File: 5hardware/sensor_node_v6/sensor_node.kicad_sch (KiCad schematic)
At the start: 71 parts, among them J1 USB_C_Receptacle_USB2.0, J2 PJ-320D-A, J3 Conn_01x18_Socket, J4 Conn_01x18_Socket, J5 Conn_01x04_Pin, P1 S3B-PH-SM4-TB, Q1 BC818, Q2 Si2371EDS, Q3 AO3400A, Q4 Si2371EDS, Q5 Si2371EDS, SW1 SW_Push, SW2 RotaryEncoder, SW3 SW_Push, SW4 SW_Push, SW5 SW_Push, SW7 SW_Push, U1 INA219AxD, U12 APDS-9960, U13 SHT31-DIS, U15 DS1307Z+, U16 DS3231M, U17 BH1750FVI-TR, U2 ESP-12F, U4 CH32V003F4P6, U7 XC6206PxxxMR, U8 TPL5110, Y1 Crystal, Y2 Crystal

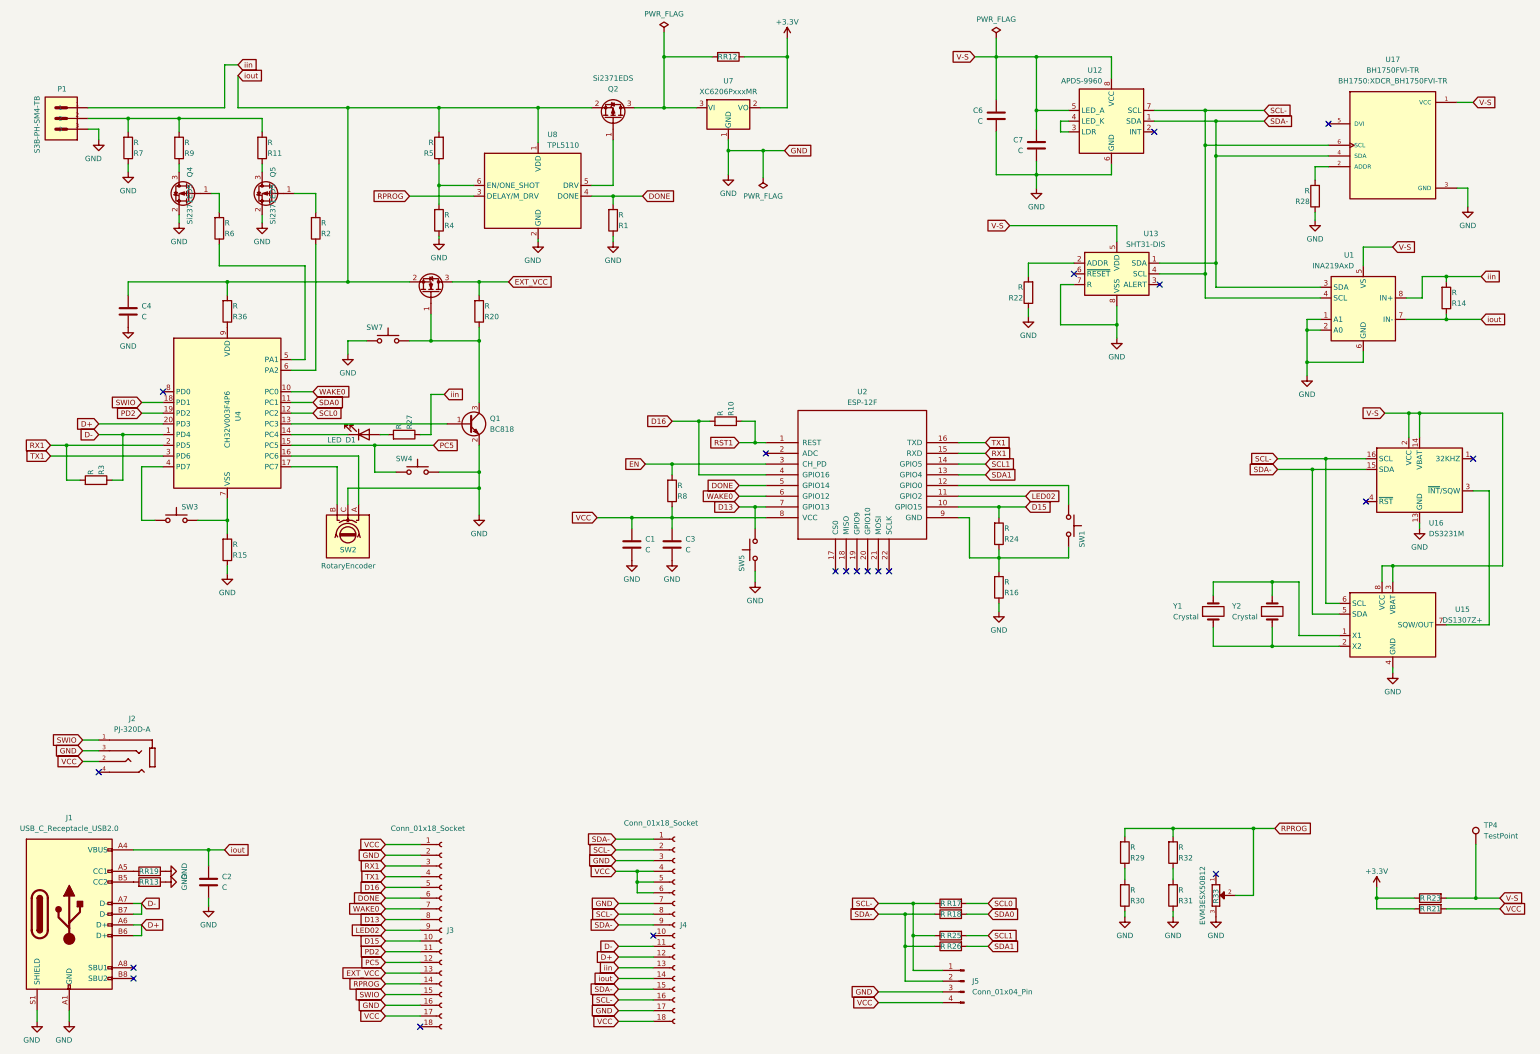
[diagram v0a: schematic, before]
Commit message: update PCB v8.0
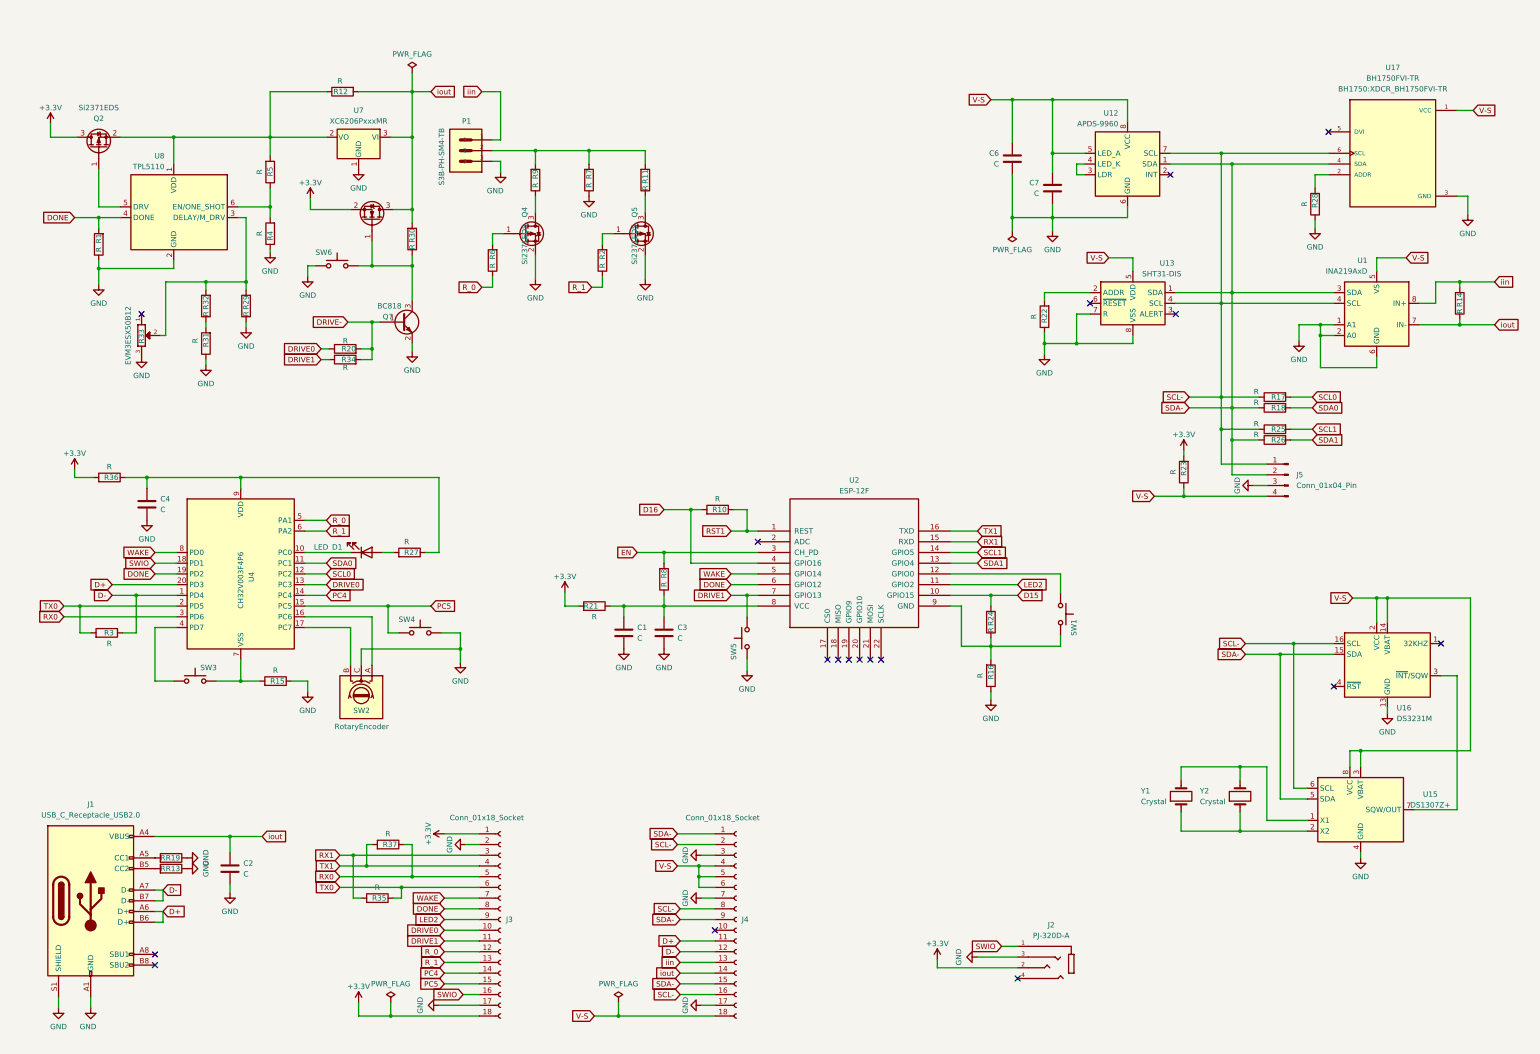
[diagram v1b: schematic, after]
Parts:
- removed Q1: BC818, Package_TO_SOT_SMD:SOT-23, symbol Transistor_BJT:BC818
- removed Q3: AO3400A, Package_TO_SOT_SMD:SOT-23, symbol Transistor_FET:AO3400A
- removed SW7: SW_Push, Button_Switch_SMD:SW_SPST_PTS810, symbol Switch:SW_Push
- removed TP4: TestPoint, Connector_PinHeader_1.00mm:PinHeader_1x01_P1.00mm_Vertical, symbol Connector:TestPoint
- added Q6: AO3400A, Package_TO_SOT_SMD:SOT-23, symbol Transistor_FET:AO3400A
- added Q7: BC818, Package_TO_SOT_SMD:SOT-23, symbol Transistor_BJT:BC818
- added R34, R35, R37: R, Resistor_SMD:R_0603_1608Metric, symbol Device:R
- added SW6: SW_Push, Button_Switch_SMD:SW_SPST_PTS810, symbol Switch:SW_Push
- C1, C2, C3, C4, C6, C7: footprint Capacitor_SMD:C_0805_2012Metric -> Capacitor_SMD:C_0603_1608Metric
- R1, R11, R13, R19, R2, R20, R24, R27, R29, R3, R30, R6, R7, R8, R9: footprint Resistor_SMD:R_0805_2012Metric -> Resistor_SMD:R_0603_1608Metric
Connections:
- net +3.3V: now also J2.2, J3.1 (Pin_1), J3.18 (Pin_18), Q2.3 (D), R21.2, R23.2, R36.2, Q6.2 (S); no longer R12.1, R21.1, R23.1, U7.2 (VO)
- net D+: now also J4.11 (Pin_11); no longer J4.12 (Pin_12)
- net D-: now also J4.12 (Pin_12); no longer J4.11 (Pin_11)
- net D15: no longer J3.10 (Pin_10)
- net D16: no longer J3.5 (Pin_5)
- net DONE: now also J3.8 (Pin_8), U2.6 (GPIO12), U4.19 (PD2); no longer J3.6 (Pin_6), U2.5 (GPIO14)
- net GND: now also J3.17 (Pin_17), R29.1, Q7.2 (E), SW6.1; no longer J3.16 (Pin_16), R30.1
- net PC5: now also J3.15 (Pin_15); no longer J3.12 (Pin_12)
- net RX1: now also R35.2; no longer R3.2, U4.2 (PD5)
- net SWIO: now also J3.16 (Pin_16); no longer J3.15 (Pin_15)
- net TX1: now also R37.2; no longer U4.3 (PD6)
- net V-S: now also J4.18 (Pin_18), J4.4 (Pin_4), J4.5 (Pin_5), J4.6 (Pin_6), J5.4 (Pin_4), R23.1; no longer R23.2
- net iin: no longer R27.1
- net iout: now also R12.2, R30.2, U7.3 (VI), Q6.3 (D); no longer C4.1, Q2.2 (S), R36.2, R5.2, U8.1 (VDD)
- net R_1: now reaches R2.1, U4.6 (PA2)
- net R_1: now also J3.13 (Pin_13)
- net DRIVE0: now reaches U4.13 (PC3)
- net DRIVE0: now also J3.10 (Pin_10), R20.1
- net at D1.1 (K): now also U4.10 (PC0); no longer U4.14 (PC4)
- net R_0: now reaches R6.1, U4.5 (PA1)
- net R_0: now also J3.12 (Pin_12)
- net WAKE: now reaches U4.8 (PD0)
- net WAKE: now also J3.7 (Pin_7), U2.5 (GPIO14)
- net at R36.1, U4.9 (VDD): now also C4.1, R27.1
- net D13 renamed DRIVE1
- net DRIVE1: now also J3.11 (Pin_11), R34.1; no longer J3.8 (Pin_8)
- net EXT_VCC renamed DRIVE-
- net DRIVE-: now also Q7.1 (B), R34.2; no longer J3.13 (Pin_13)
- net LED02 renamed LED2
- removed net PD2: J3.11 (Pin_11), U4.19 (PD2)
- net RPROG: no longer names the net of R29.2, R32.2, R33.2, U8.3 (DELAY/M_DRV)
- net RPROG: no longer J3.14 (Pin_14)
- removed net VCC: C1.1, C3.1, J2.2, J3.1 (Pin_1), J3.17 (Pin_17), J4.18 (Pin_18), J4.4 (Pin_4), J4.5 (Pin_5), J4.6 (Pin_6), J5.4 (Pin_4), R21.2, R8.1, U2.8 (VCC)
- removed net WAKE0: J3.7 (Pin_7), U2.6 (GPIO12), U4.10 (PC0)
- new net: C1.1, C3.1, R21.1, R8.1, U2.8 (VCC)
- new net: Q2.2 (S), R12.1, R5.2, U7.2 (VO), U8.1 (VDD)
- new net: Q6.1 (G), Q7.3 (C), R30.1, SW6.2
- new net PC4: J3.14 (Pin_14), U4.14 (PC4)
- new net RX0: J3.5 (Pin_5), R37.1, U4.3 (PD6)
- new net TX0: J3.6 (Pin_6), R3.2, R35.1, U4.2 (PD5)
- no-connect marks 20 -> 18
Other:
- moved on the sheet: C1, C2, C3, C4, C6, C7, D1, J1, J2, J3, J4, J5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
